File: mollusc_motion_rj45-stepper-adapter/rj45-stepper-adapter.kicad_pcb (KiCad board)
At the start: 2 copper layers, 33 x 24.1 mm, 3 parts, among them J2 Conn_01x03, J3 RJ45_Shielded, J6 Conn_01x06

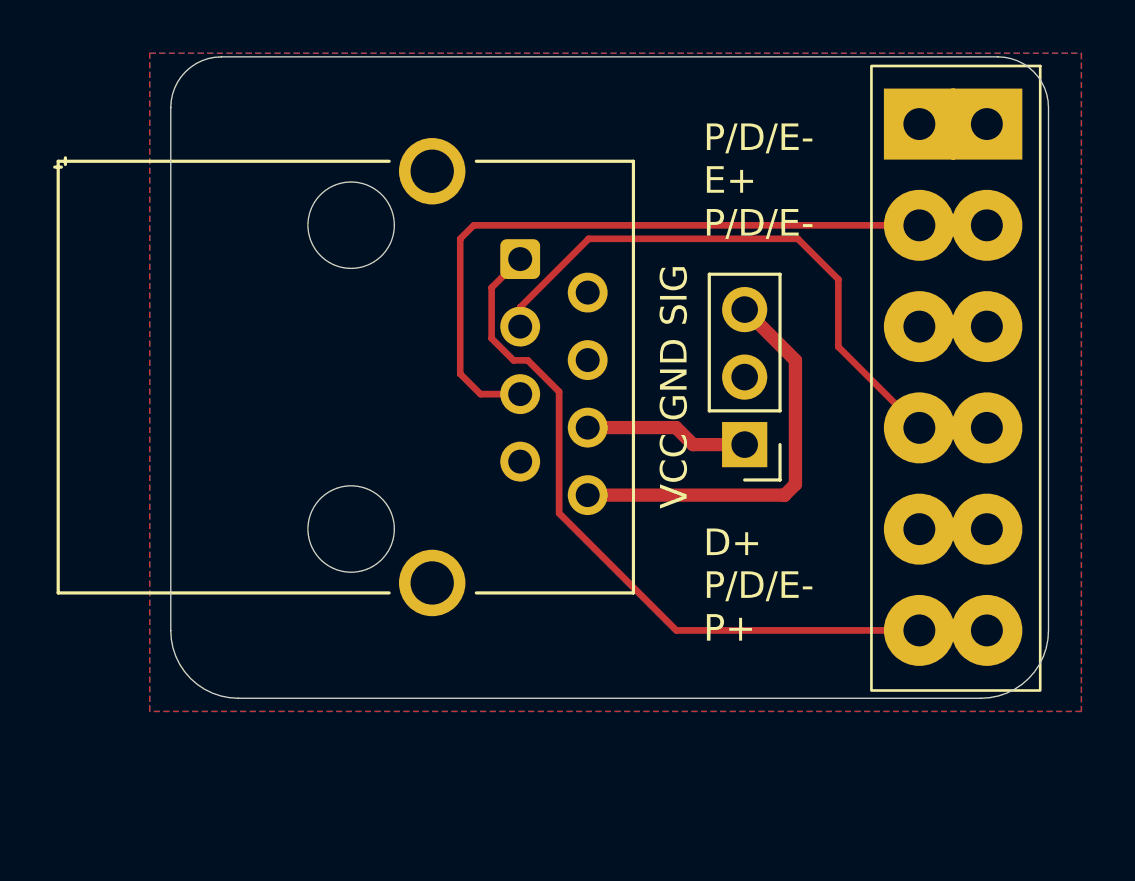
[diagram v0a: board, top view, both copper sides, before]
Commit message: v3
in production
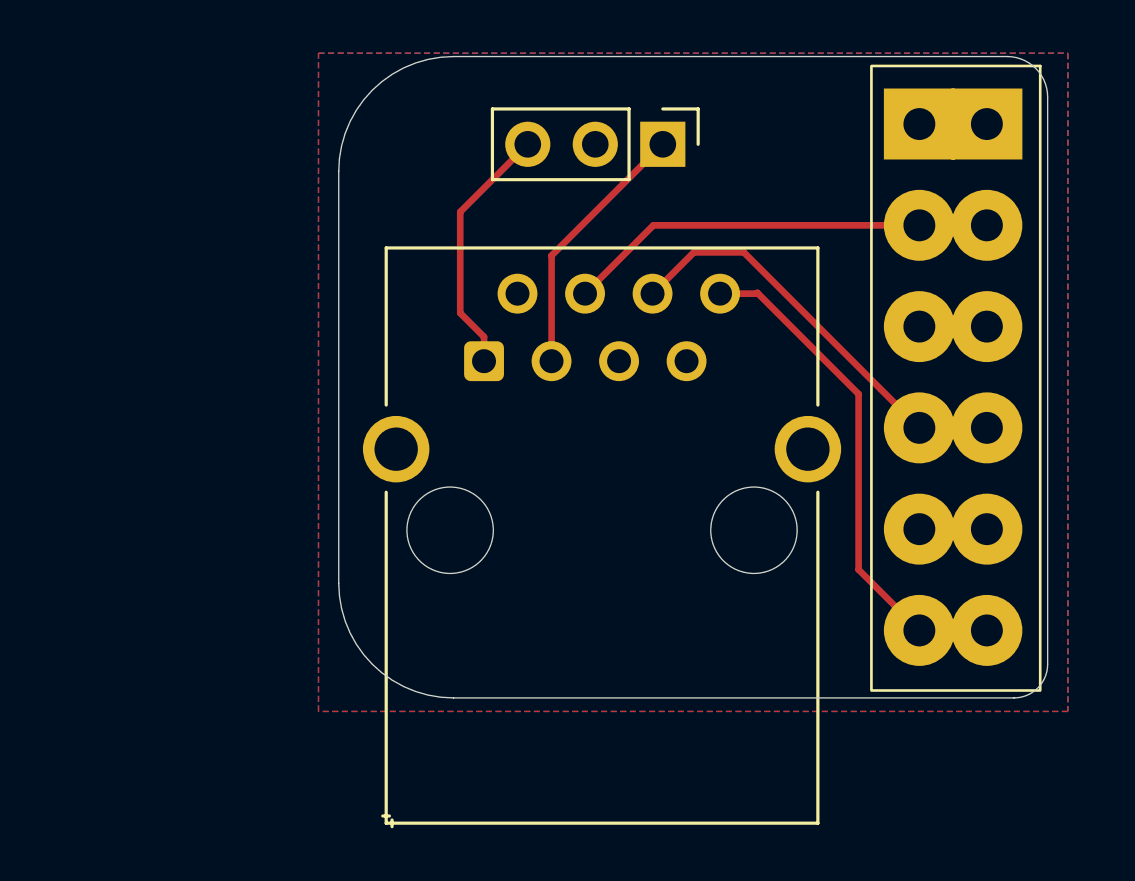
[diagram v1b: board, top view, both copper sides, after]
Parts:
- added G***: LOGO, LOGO, B.Cu at (150.1, 114.6)
- moved J3 12.0 mm to (144.9, 113.1), turned to 0 degrees
- moved J2 11.7 mm to (152.9, 98.6), turned to -90 degrees
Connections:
- J2 pad 1: /3.3V -> /VCC 3.3V
- J3 pad 1: /PUL+ -> /SIG
- J3 pad 2: /P-, D-, E- -> GND
- J3 pad 3: /DIR+ -> /VCC 3.3V
- J3 pad 4: /P-, D-, E- -> /ENA+
- J3 pad 5: /ENA+ -> GND
- J3 pad 6: /3.3V -> /DIR+
- J3 pad 8: /SIG -> /PUL+
- J6 pad 1: /P-, D-, E- -> GND
- J6 pad 3: /P-, D-, E- -> GND
- J6 pad 5: /P-, D-, E- -> GND
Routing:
- net /ENA+: track 25.1 -> 13.6 mm
- net /VCC 3.3V: track 0.00 -> 9.89 mm
- net /PUL+: track 26.8 -> 17.0 mm
- net /DIR+: track 21.2 -> 13.4 mm
- net /3.3V: track 6.17 -> 0.00 mm
- net /SIG: track 15.4 -> 9.58 mm
- added copper zone on F.Cu, net GND
- removed copper zone on F.Cu, net /P-, D-, E-
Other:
- board size 33 x 24.1 mm -> 26.7 x 24.1 mm
- board text added: "DIR+"
- board text added: "ENA+"
- board text added: "GND"
- board text added: "PUL+"
- board text removed: "- E+ - D+ - P+"
- board text removed: "D+ P/D/E- P+"
- board text removed: "P/D/E- E+ P/D/E-"
